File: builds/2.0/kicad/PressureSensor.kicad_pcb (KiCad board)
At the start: 2 copper layers, 38.1 x 57.2 mm, 22 parts, among them J1 PROG, U1 SENSOR, U2 HX710, U3 DISPLAY, U4 AVR64DD32

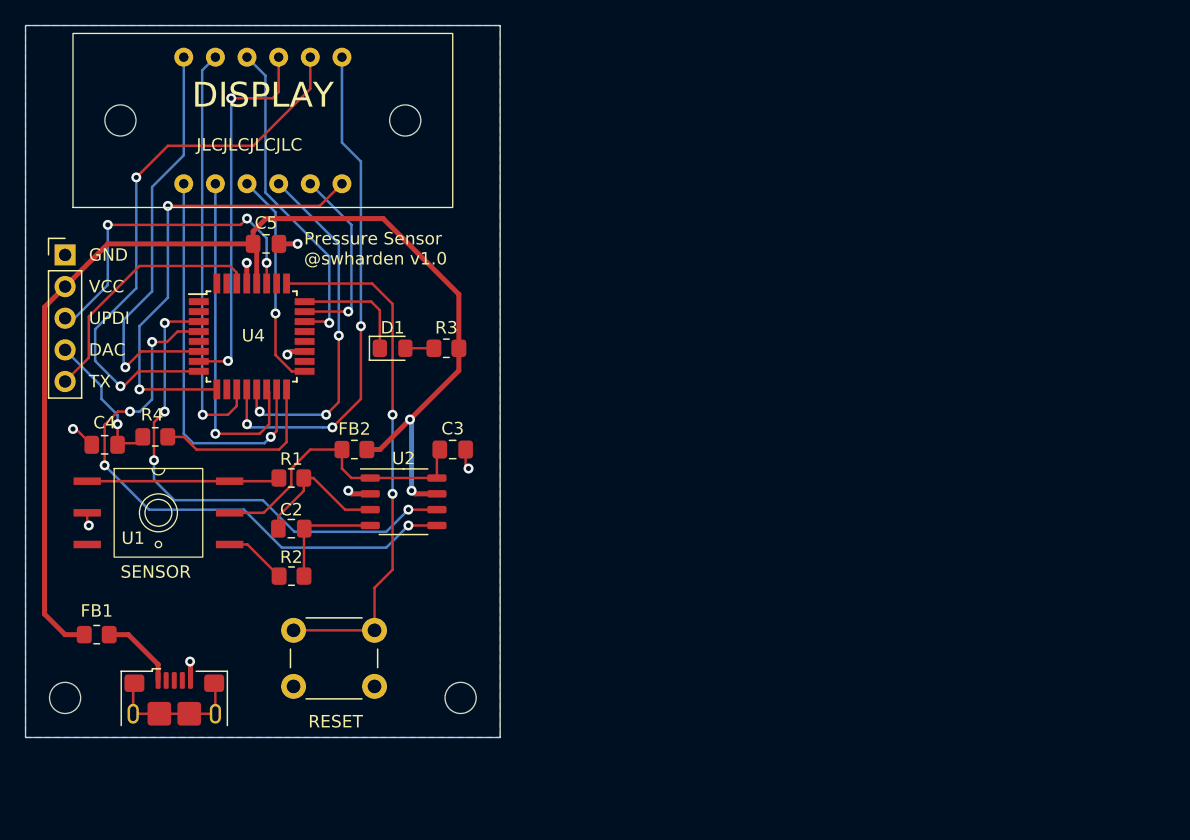
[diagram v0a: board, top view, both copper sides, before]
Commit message: update libraries
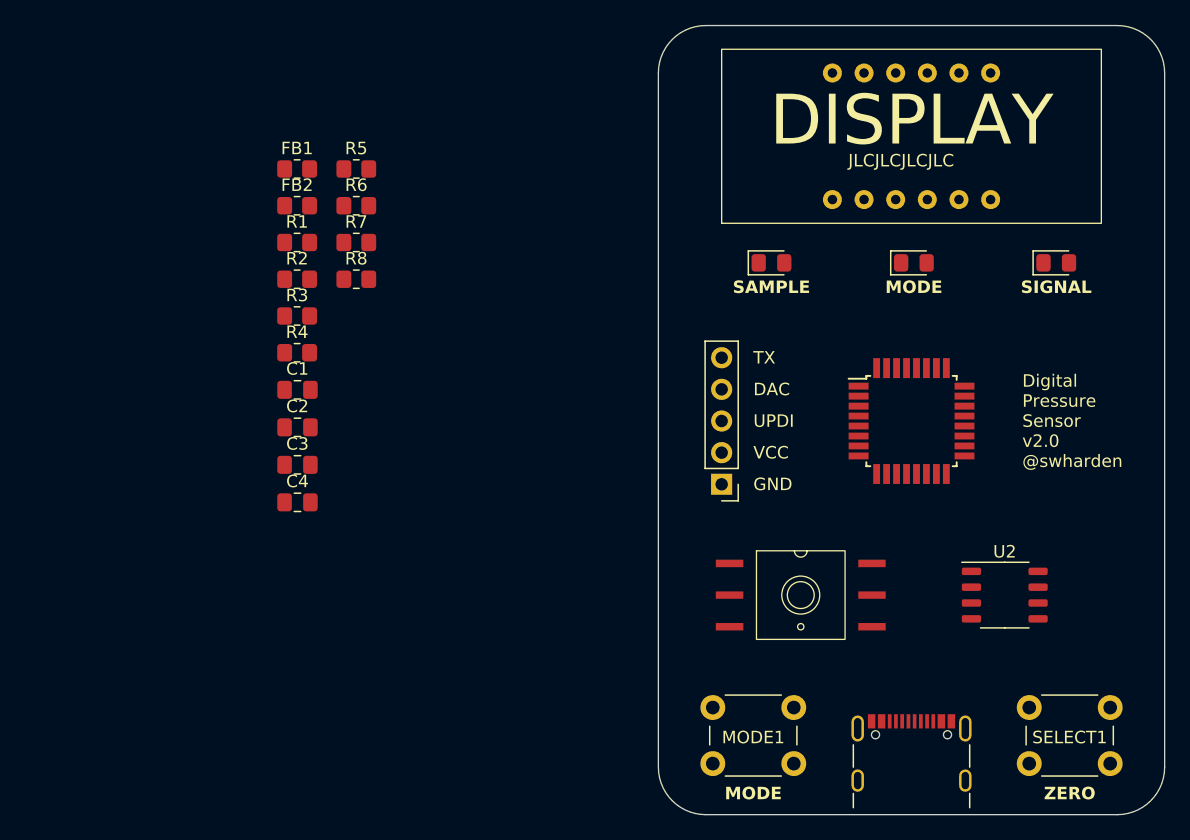
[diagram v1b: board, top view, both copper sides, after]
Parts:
- removed C5: .1u, Capacitor_SMD:C_0805_2012Metric_Pad1.18x1.45mm_HandSolder
- removed POWER: USB_B_Micro, Connector_USB:USB_Micro-B_Amphenol_10118193-0001LF_Horizontal
- removed REF** (x4): MountingHole_2.5mm, MountingHole:MountingHole_2.5mm
- removed RESET: SW_Push, Button_Switch_THT:SW_PUSH_6mm_H5mm
- added C1: .1u, Capacitor_SMD:C_0805_2012Metric_Pad1.18x1.45mm_HandSolder, F.Cu at (123.4, 80.0)
- added D2: MODE, LED_SMD:LED_0805_2012Metric_Pad1.15x1.40mm_HandSolder, F.Cu at (172.9, 69.8)
- added D3: STATUS, LED_SMD:LED_0805_2012Metric_Pad1.15x1.40mm_HandSolder, F.Cu at (161.5, 69.8)
- added J2: PROG, Connector_PinHeader_2.54mm:PinHeader_1x05_P2.54mm_Vertical, F.Cu at (157.5, 87.6)
- added MODE1: SW_Push, Button_Switch_THT:SW_PUSH_6mm_H5mm, F.Cu at (156.8, 105.5)
- added R5: 100k, Resistor_SMD:R_0805_2012Metric_Pad1.20x1.40mm_HandSolder, F.Cu at (128.2, 62.3)
- added R6: 100k, Resistor_SMD:R_0805_2012Metric_Pad1.20x1.40mm_HandSolder, F.Cu at (128.2, 65.3)
- added R7: 100k, Resistor_SMD:R_0805_2012Metric_Pad1.20x1.40mm_HandSolder, F.Cu at (128.2, 68.2)
- added R8: 1k, Resistor_SMD:R_0805_2012Metric_Pad1.20x1.40mm_HandSolder, F.Cu at (128.2, 71.2)
- added SELECT1: SW_Push, Button_Switch_THT:SW_PUSH_6mm_H5mm, F.Cu at (182.2, 105.5)
- D1: value STATUS -> SAMPLE
- J1: value PROG -> USB_C_Receptacle_PowerOnly_6P; footprint Connector_PinHeader_2.54mm:PinHeader_1x05_P2.54mm_Vertical -> AAA_CUSTOM_LIBRARY:USB_C_Receptacle_GCT_USB4105-xx-A_16P_TopMnt_Horizontal
- R1, R2: value 1k -> 5.7k
- R3: value 10k -> 1k
- U1: footprint Library:pressure-sensor-SOIC-6 -> AAA_CUSTOM_LIBRARY:pressure-sensor-SOIC-6
- U3: footprint Library:7_seg_display_DIP12 -> AAA_CUSTOM_LIBRARY:7_seg_display_DIP12
- moved J1 79.4 mm to (172.7, 110.3)
- moved D1 53.7 mm to (184.3, 69.8)
- moved U4 53.4 mm to (172.7, 82.5)
- moved U3 52.1 mm to (172.7, 59.7)
- moved U1 52.0 mm to (163.8, 96.5)
- moved U2 48.8 mm to (180.2, 96.5)
- moved FB1 40.7 mm to (123.4, 62.3), turned to 0 degrees
- moved R2 23.8 mm to (123.4, 71.2), turned to 0 degrees
- moved FB2 20.1 mm to (123.4, 65.3)
- moved R1 18.9 mm to (123.4, 68.2)
- moved C4 16.2 mm to (123.4, 89.1), turned to 0 degrees
- moved R4 13.2 mm to (123.4, 77.1), turned to 0 degrees
- moved C3 12.5 mm to (123.4, 86.1)
- moved R3 12.3 mm to (123.4, 74.1)
- moved C2 8.15 mm to (123.4, 83.1)
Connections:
- C2 pad 1: Net-(U2-IN_NEG) -> AVCC
- C2 pad 2: Net-(U2-IN_POS) -> GND
- C3 pad 1: AVCC -> VCC
- D1 pad 1: Net-(D1-K) -> LED1
- FB1 pad 1: Net-(C1-VBUS) -> Net-(FB1-Pad1)
- R1 pad 1: Net-(R1-Pad1) -> Net-(J1-CC1)
- R1 pad 2: Net-(U2-IN_NEG) -> GND
- R2 pad 1: Net-(U2-IN_POS) -> GND
- R2 pad 2: Net-(U1-Vpos) -> Net-(J1-CC2)
- R3 pad 1: Net-(D1-A) -> Net-(R3-Pad1)
- R3 pad 2: VCC -> Net-(U2-IN_NEG)
- R4 pad 1: Net-(U4-PD6) -> Net-(U2-IN_POS)
- R4 pad 2: DAC -> Net-(U1-Vpos)
- U1 pad 1: Net-(R1-Pad1) -> Net-(R3-Pad1)
- U1 pad 6: Net-(R1-Pad1) -> Net-(R3-Pad1)
- U4 pad 1: unconnected-(U4-PA3-Pad1) -> LED2
- U4 pad 16: Net-(U4-PD6) -> MCU_DAC
- U4 pad 19: GND -> unconnected-(U4-AGND-Pad19)
- U4 pad 2: unconnected-(U4-PA4-Pad2) -> LED3
- U4 pad 24: Net-(D1-K) -> BTN1
- U4 pad 25: Net-(U4-PF5) -> BTN2
- U4 pad 32: unconnected-(U4-PA2-Pad32) -> LED1
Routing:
- net VCC: track 95.2 -> 0.00 mm, vias 2 -> 0
- net SPI_CLK: track 46.8 -> 0.00 mm, vias 4 -> 0
- net DIG_3: track 45.2 -> 0.00 mm, vias 2 -> 0
- net Net-(U4-PF5): track 42.5 -> 0.00 mm, vias 2 -> 0
- net SEG_B: track 41.1 -> 0.00 mm, vias 3 -> 0
- net SPI_MISO: track 40.9 -> 0.00 mm, vias 4 -> 0
- net DIG_4: track 36.6 -> 0.00 mm, vias 2 -> 0
- net SEG_A: track 33.5 -> 0.00 mm, vias 1 -> 0
- net DIG_1: track 33.4 -> 0.00 mm, vias 1 -> 0
- net SEG_E: track 31.6 -> 0.00 mm, vias 1 -> 0
- net DIG_2: track 30.4 -> 0.00 mm, vias 2 -> 0
- net SEG_C: track 28.3 -> 0.00 mm, vias 3 -> 0
- net SEG_D: track 27.6 -> 0.00 mm, vias 1 -> 0
- net UPDI: track 26.6 -> 0.00 mm, vias 3 -> 0
- net SEG_F: track 26.1 -> 0.00 mm, vias 1 -> 0
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- removed copper zone on B.Cu, net GND
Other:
- board size 38.1 x 57.2 mm -> 40.6 x 63.3 mm
- board text added: "Digital Pressure Sensor v2.0 @swharden"
- board text added: "MODE"
- board text added: "SAMPLE"
- board text added: "SIGNAL"
- board text added: "ZERO"
- board text removed: "Pressure Sensor @swharden v1.0"
- board text removed: "SENSOR"
